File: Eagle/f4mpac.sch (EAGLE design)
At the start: 51 parts, among them CN1 DIP40 MB CONN, IC1 YM2413, IC10 27C256L, IC2 74LS30D, IC3 74LS04D, IC4 LM4558N, IC5 Z80, IC6 74LS30D, IC7 74LS02D, IC8 74LS74D, IC9 74LS125D

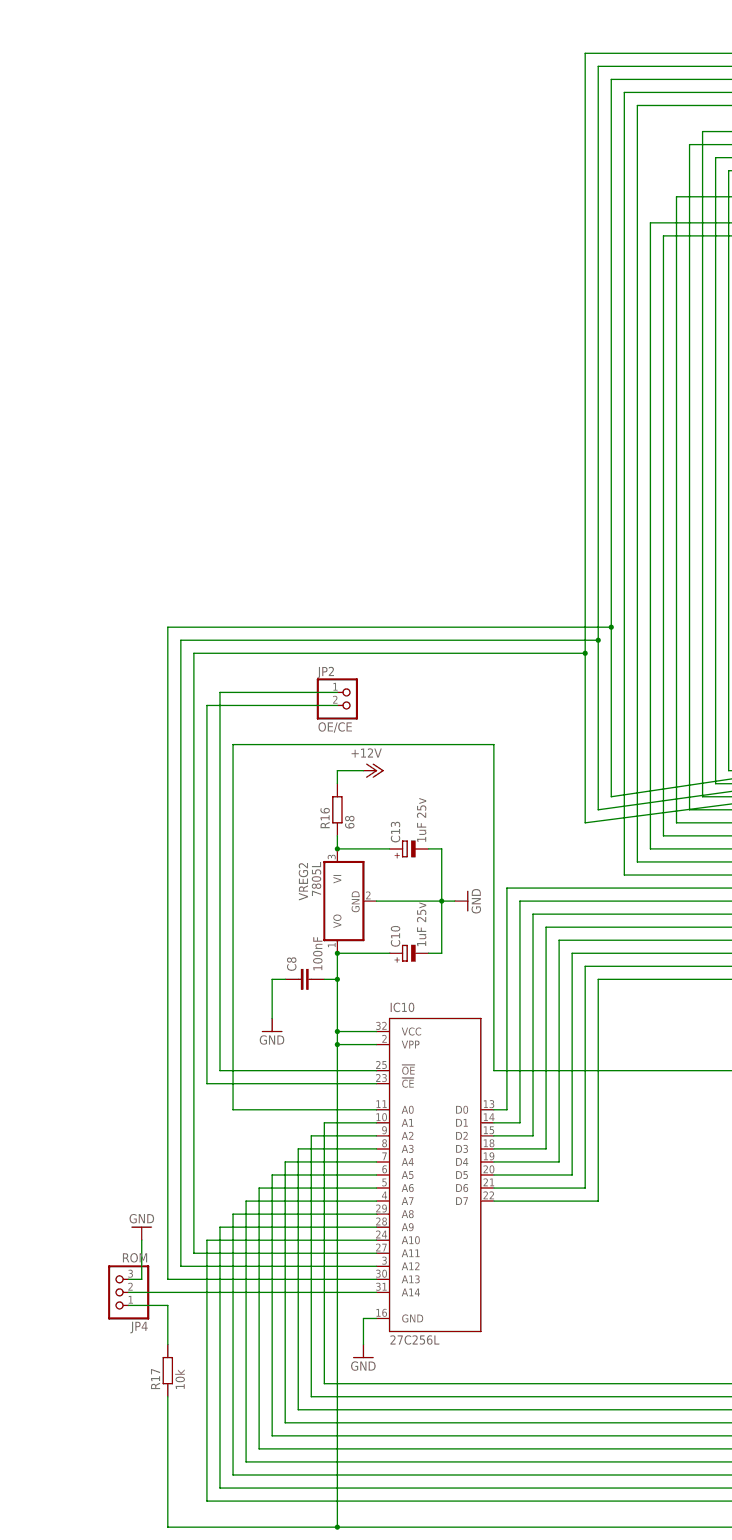
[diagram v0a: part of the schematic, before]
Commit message: Updated source and gerber files, added schematics
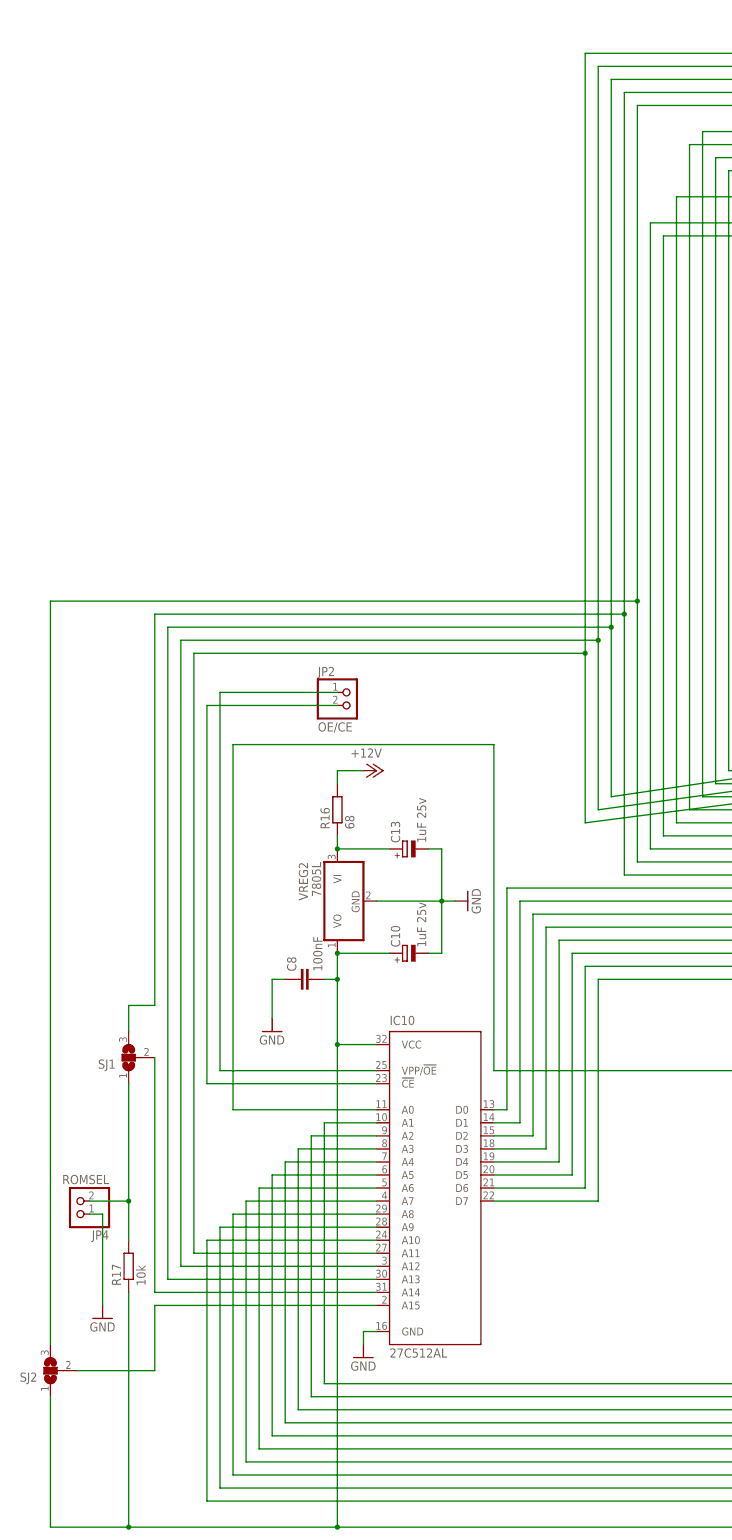
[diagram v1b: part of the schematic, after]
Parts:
- added SJ1, SJ2: (no value), jumper:SJ2W
- IC10: value 27C256L -> 27C512AL; device microchip:27C256L -> microchip:27C512AL
- JP4: value ROM -> ROMSEL; device pinhead:PINHD-1X3/90 -> pinhead:PINHD-1X2/90
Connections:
- new net N$10: IC10.A14, SJ1.2
- net +5VREG: now also SJ2.1; no longer IC10.VPP
- net A14: now also SJ1.3
- net A15: now also SJ2.3
- net GND: now also JP4.1; no longer JP4.3
- net N$20: now also IC10.VPP/!OE; no longer IC10.!OE
- net N$25: now also IC10.A15, SJ2.2; no longer IC10.A14, JP4.2
- net N$26: now also JP4.2, SJ1.1; no longer JP4.1
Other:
- moved on the sheet: IC10, R17
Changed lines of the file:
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@@
 <part name="GND12" library="supply1" deviceset="GND" device=""/>
 <part name="C14" library="rcl" deviceset="C-EU" device="C0805" value="1nF"/>
-<part name="IC10" library="microchip" deviceset="27*256" device="L" technology="C"/>
-<part name="R17" library="rcl" deviceset="R-EU_" device="R0805" value="10k"/>
-<part name="JP4" library="pinhead" deviceset="PINHD-1X3" device="/90" value="ROM"/>
-<part name="GND13" library="supply1" deviceset="GND" device=""/>
 <part name="C15" library="rcl" deviceset="C-EU" device="C0805" value="100nF"/>
 <part name="GND14" library="supply1" deviceset="GND" device=""/>
 <part name="C16" library="rcl" deviceset="C-EU" device="C0805" value="1nF"/>
+<part name="IC10" library="microchip" deviceset="27*512A" device="L" technology="C"/>
+<part name="SJ2" library="jumper" deviceset="SJ2W" device=""/>
+<part name="SJ1" library="jumper" deviceset="SJ2W" device=""/>
+<part name="JP4" library="pinhead" deviceset="PINHD-1X2" device="/90" value="ROMSEL"/>
+<part name="GND13" library="supply1" deviceset="GND" device=""/>
+<part name="R17" library="rcl" deviceset="R-EU_" device="R0805" value="10k"/>
 </parts>
 <sheets>
@@
 <instance part="GND12" gate="1" x="-129.54" y="48.26"/>
 <instance part="C14" gate="G$1" x="172.72" y="76.2" rot="R90"/>
-<instance part="IC10" gate="G$1" x="-99.06" y="20.32"/>
-<instance part="R17" gate="G$1" x="-149.86" y="-17.78" rot="R90"/>
-<instance part="JP4" gate="A" x="-160.02" y="-2.54" rot="R180"/>
-<instance part="GND13" gate="1" x="-154.94" y="10.16" rot="R180"/>
 <instance part="C15" gate="G$1" x="81.28" y="22.86" rot="R180"/>
 <instance part="GND14" gate="1" x="81.28" y="15.24"/>
 <instance part="C16" gate="G$1" x="167.64" y="12.7" rot="R90"/>
+<instance part="IC10" gate="G$1" x="-99.06" y="17.78"/>
+<instance part="SJ2" gate="G$1" x="-172.72" y="-17.78" rot="R180"/>
+<instance part="SJ1" gate="G$1" x="-157.48" y="43.18" rot="R180"/>
+<instance part="JP4" gate="G$1" x="-167.64" y="15.24" rot="R180"/>
+<instance part="GND13" gate="1" x="-162.56" y="-7.62"/>
+<instance part="R17" gate="G$1" x="-157.48" y="2.54" rot="R90"/>
 </instances>
 <busses>
@@
 </segment>
 <segment>
-<pinref part="IC10" gate="G$1" pin="GND"/>
-<pinref part="GND10" gate="1" pin="GND"/>
-<wire x1="-109.22" y1="-7.62" x2="-111.76" y2="-7.62" width="0.1524" layer="91"/>
-<wire x1="-111.76" y1="-7.62" x2="-111.76" y2="-12.7" width="0.1524" layer="91"/>
-</segment>
-<segment>
-<pinref part="JP4" gate="A" pin="3"/>
-<wire x1="-157.48" y1="0" x2="-154.94" y2="0" width="0.1524" layer="91"/>
-<wire x1="-154.94" y1="0" x2="-154.94" y2="7.62" width="0.1524" layer="91"/>
-<pinref part="GND13" gate="1" pin="GND"/>
-</segment>
-<segment>
 <pinref part="GND14" gate="1" pin="GND"/>
 <pinref part="C15" gate="G$1" pin="1"/>
 <wire x1="81.28" y1="17.78" x2="81.28" y2="20.32" width="0.1524" layer="91"/>
+</segment>
+<segment>
+<pinref part="IC10" gate="G$1" pin="GND"/>
+<pinref part="GND10" gate="1" pin="GND"/>
+<wire x1="-109.22" y1="-10.16" x2="-111.76" y2="-10.16" width="0.1524" layer="91"/>
+<wire x1="-111.76" y1="-10.16" x2="-111.76" y2="-12.7" width="0.1524" layer="91"/>
+</segment>
+<segment>
+<pinref part="JP4" gate="G$1" pin="1"/>
+<wire x1="-165.1" y1="12.7" x2="-162.56" y2="12.7" width="0.1524" layer="91"/>
+<wire x1="-162.56" y1="12.7" x2="-162.56" y2="-5.08" width="0.1524" layer="91"/>
+<pinref part="GND13" gate="1" pin="GND"/>
 </segment>
 </net>
@@
 <wire x1="0" y1="104.14" x2="0" y2="81.28" width="0.1524" layer="91"/>
 <wire x1="0" y1="81.28" x2="-58.42" y2="81.28" width="0.1524" layer="91"/>
-<wire x1="-58.42" y1="81.28" x2="-58.42" y2="228.6" width="0.1524" layer="91"/>
 <pinref part="CN1" gate="G$1" pin="5"/>
+<wire x1="-58.42" y1="81.28" x2="-58.42" y2="132.08" width="0.1524" layer="91"/>
+<wire x1="-58.42" y1="132.08" x2="-58.42" y2="228.6" width="0.1524" layer="91"/>
 <wire x1="-58.42" y1="228.6" x2="-5.08" y2="228.6" width="0.1524" layer="91"/>
+<wire x1="-58.42" y1="132.08" x2="-172.72" y2="132.08" width="0.1524" layer="91"/>
+<wire x1="-172.72" y1="132.08" x2="-172.72" y2="-12.7" width="0.1524" layer="91"/>
+<junction x="-58.42" y="132.08"/>
+<pinref part="SJ2" gate="G$1" pin="3"/>
 </segment>
 </net>
@@
 <wire x1="2.54" y1="104.14" x2="2.54" y2="78.74" width="0.1524" layer="91"/>
 <wire x1="2.54" y1="78.74" x2="-60.96" y2="78.74" width="0.1524" layer="91"/>
-<wire x1="-60.96" y1="78.74" x2="-60.96" y2="231.14" width="0.1524" layer="91"/>
+<wire x1="-60.96" y1="78.74" x2="-60.96" y2="129.54" width="0.1524" layer="91"/>
 <pinref part="CN1" gate="G$1" pin="4"/>
+<wire x1="-60.96" y1="129.54" x2="-60.96" y2="231.14" width="0.1524" layer="91"/>
 <wire x1="-60.96" y1="231.14" x2="-5.08" y2="231.14" width="0.1524" layer="91"/>
+<wire x1="-60.96" y1="129.54" x2="-152.4" y2="129.54" width="0.1524" layer="91"/>
+<wire x1="-152.4" y1="129.54" x2="-152.4" y2="53.34" width="0.1524" layer="91"/>
+<junction x="-60.96" y="129.54"/>
+<pinref part="SJ1" gate="G$1" pin="3"/>
+<wire x1="-152.4" y1="53.34" x2="-157.48" y2="53.34" width="0.1524" layer="91"/>
+<wire x1="-157.48" y1="53.34" x2="-157.48" y2="48.26" width="0.1524" layer="91"/>
 </segment>
 </net>
@@
 <wire x1="-116.84" y1="-48.26" x2="-116.84" y2="45.72" width="0.1524" layer="91"/>
 <pinref part="VREG2" gate="A1" pin="VO"/>
-<wire x1="-116.84" y1="45.72" x2="-116.84" y2="48.26" width="0.1524" layer="91"/>
-<wire x1="-116.84" y1="48.26" x2="-116.84" y2="58.42" width="0.1524" layer="91"/>
+<wire x1="-116.84" y1="45.72" x2="-116.84" y2="58.42" width="0.1524" layer="91"/>
 <wire x1="-116.84" y1="63.5" x2="-116.84" y2="58.42" width="0.1524" layer="91"/>
 <pinref part="C10" gate="G$1" pin="+"/>
@@
 <junction x="-116.84" y="58.42"/>
 <pinref part="IC10" gate="G$1" pin="VCC"/>
-<wire x1="-116.84" y1="48.26" x2="-109.22" y2="48.26" width="0.1524" layer="91"/>
-<junction x="-116.84" y="48.26"/>
-<pinref part="IC10" gate="G$1" pin="VPP"/>
-<wire x1="-116.84" y1="45.72" x2="-109.22" y2="45.72" width="0.1524" layer="91"/>
+<wire x1="-109.22" y1="45.72" x2="-116.84" y2="45.72" width="0.1524" layer="91"/>
 <junction x="-116.84" y="45.72"/>
+<wire x1="-172.72" y1="-48.26" x2="-157.48" y2="-48.26" width="0.1524" layer="91"/>
+<junction x="-116.84" y="-48.26"/>
+<pinref part="SJ2" gate="G$1" pin="1"/>
+<wire x1="-157.48" y1="-48.26" x2="-116.84" y2="-48.26" width="0.1524" layer="91"/>
+<wire x1="-172.72" y1="-22.86" x2="-172.72" y2="-48.26" width="0.1524" layer="91"/>
 <pinref part="R17" gate="G$1" pin="1"/>
-<wire x1="-116.84" y1="-48.26" x2="-149.86" y2="-48.26" width="0.1524" layer="91"/>
-<wire x1="-149.86" y1="-48.26" x2="-149.86" y2="-22.86" width="0.1524" layer="91"/>
-<junction x="-116.84" y="-48.26"/>
+<wire x1="-157.48" y1="-2.54" x2="-157.48" y2="-48.26" width="0.1524" layer="91"/>
+<junction x="-157.48" y="-48.26"/>
 </segment>
 </net>
@@
 <wire x1="-139.7" y1="114.3" x2="-139.7" y2="40.64" width="0.1524" layer="91"/>
 <wire x1="-139.7" y1="40.64" x2="-109.22" y2="40.64" width="0.1524" layer="91"/>
-<pinref part="IC10" gate="G$1" pin="!OE"/>
+<pinref part="IC10" gate="G$1" pin="VPP/!OE"/>
 </segment>
 </net>
@@
 </segment>
 </net>
-<net name="N$25" class="0">
-<segment>
-<pinref part="IC10" gate="G$1" pin="A14"/>
-<wire x1="-109.22" y1="-2.54" x2="-157.48" y2="-2.54" width="0.1524" layer="91"/>
-<pinref part="JP4" gate="A" pin="2"/>
-</segment>
-</net>
-<net name="N$26" class="0">
-<segment>
-<pinref part="JP4" gate="A" pin="1"/>
-<pinref part="R17" gate="G$1" pin="2"/>
-<wire x1="-157.48" y1="-5.08" x2="-149.86" y2="-5.08" width="0.1524" layer="91"/>
-<wire x1="-149.86" y1="-5.08" x2="-149.86" y2="-12.7" width="0.1524" layer="91"/>
-</segment>
-</net>
 <net name="N$27" class="0">
 <segment>
@@
 </segment>
 </net>
+<net name="N$10" class="0">
+<segment>
+<pinref part="IC10" gate="G$1" pin="A14"/>
+<wire x1="-109.22" y1="-2.54" x2="-152.4" y2="-2.54" width="0.1524" layer="91"/>
+<pinref part="SJ1" gate="G$1" pin="2"/>
+<wire x1="-152.4" y1="-2.54" x2="-152.4" y2="43.18" width="0.1524" layer="91"/>
+</segment>
+</net>
+<net name="N$25" class="0">
+<segment>
+<pinref part="IC10" gate="G$1" pin="A15"/>
+<wire x1="-109.22" y1="-5.08" x2="-152.4" y2="-5.08" width="0.1524" layer="91"/>
+<wire x1="-152.4" y1="-5.08" x2="-152.4" y2="-17.78" width="0.1524" layer="91"/>
+<pinref part="SJ2" gate="G$1" pin="2"/>
+<wire x1="-152.4" y1="-17.78" x2="-167.64" y2="-17.78" width="0.1524" layer="91"/>
+</segment>
+</net>
+<net name="N$26" class="0">
+<segment>
+<pinref part="SJ1" gate="G$1" pin="1"/>
+<wire x1="-157.48" y1="38.1" x2="-157.48" y2="15.24" width="0.1524" layer="91"/>
+<pinref part="JP4" gate="G$1" pin="2"/>
+<wire x1="-165.1" y1="15.24" x2="-157.48" y2="15.24" width="0.1524" layer="91"/>
+<pinref part="R17" gate="G$1" pin="2"/>
+<wire x1="-157.48" y1="7.62" x2="-157.48" y2="15.24" width="0.1524" layer="91"/>
+<junction x="-157.48" y="15.24"/>
+</segment>
+</net>
